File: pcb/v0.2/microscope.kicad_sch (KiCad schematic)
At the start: 26 parts, among them IC1 AL8860QMP-13, J1 Conn_01x02_Socket, J3 Conn_01x03_Socket, U1 OP07CDR, U2 NE555DR, U3 L78L05_SOT89, U4 Solder Pad, U5 Solder Pad

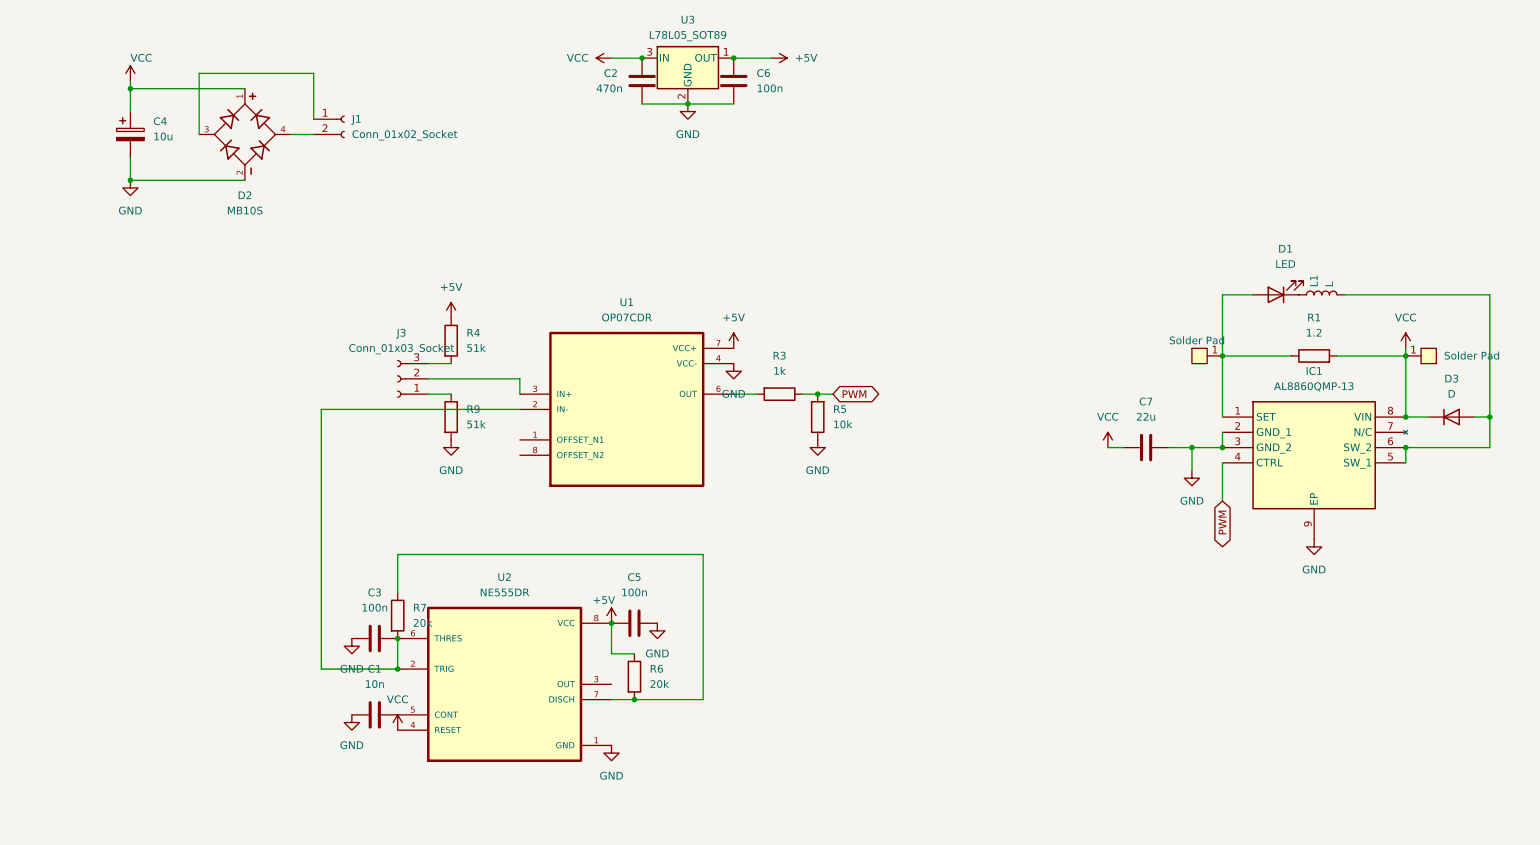
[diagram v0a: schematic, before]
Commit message: v0.2 pcb finished
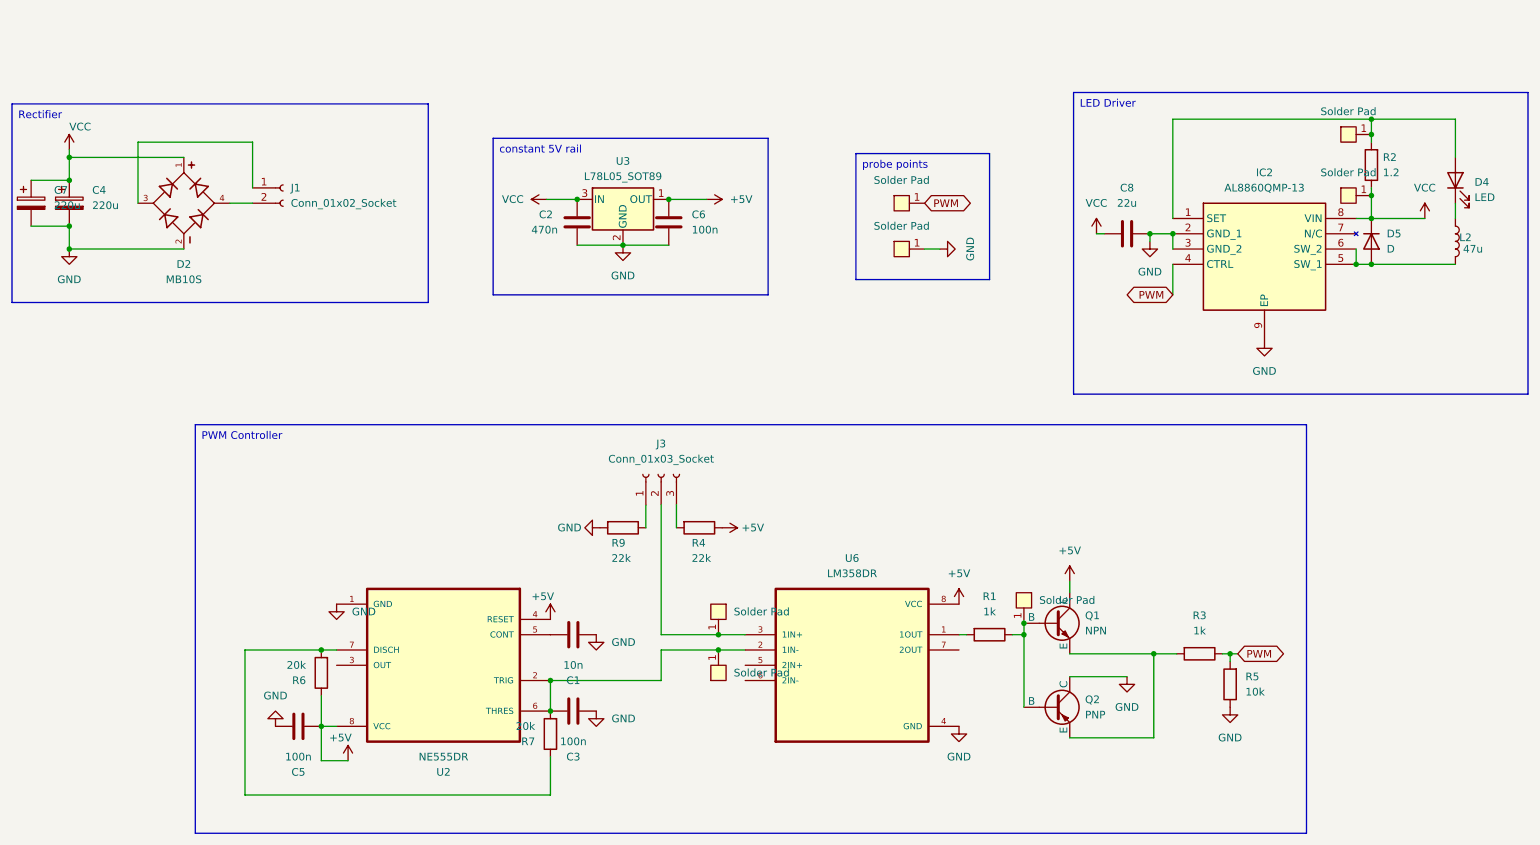
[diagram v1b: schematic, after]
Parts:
- removed C7: 22u, Capacitor_SMD:C_0805_2012Metric, symbol Device:C
- removed D1: LED, LED_SMD:LED_PLCC_2835, symbol Device:LED
- removed D3: D, Diode_SMD:D_SOD-323, symbol Device:D
- removed IC1: AL8860QMP-13, KiCad:SOP65P490X110-9N, symbol AL8860QMP-13:AL8860QMP-13
- removed L1: L, Inductor_SMD:L_1210_3225Metric, symbol Device:L
- removed U1: OP07CDR, OP07CDR:SOIC127P599X175-8N, symbol OP07CDR:OP07CDR
- added C7: 220u, Capacitor_THT:CP_Radial_D6.3mm_P2.50mm, symbol Device:C_Polarized
- added C8: 22u, Capacitor_SMD:C_0805_2012Metric, symbol Device:C
- added D4: LED, LED_SMD:LED_PLCC_2835, symbol Device:LED
- added D5: D, Diode_SMD:D_SOD-323, symbol Device:D
- added IC2: AL8860QMP-13, KiCad:SOP65P490X110-9N, symbol AL8860QMP-13:AL8860QMP-13
- added L2: 47u, Inductor_SMD:L_1210_3225Metric, symbol Device:L
- added Q1: NPN, custom_components:custom_SOT-23-3, symbol Simulation_SPICE:NPN
- added Q2: PNP, custom_components:custom_SOT-23-3, symbol Simulation_SPICE:PNP
- added R2: 1.2, Resistor_SMD:R_0603_1608Metric, symbol Device:R
- added U1, U10, U7, U8, U9: Solder Pad, custom_components:SolderPad_3x3mm, symbol custom_components:SolderPad
- added U6: LM358DR, LM358DR:SOIC127P599X175-8N, symbol LM358DR:LM358DR
- C1, C2, C3, C5, C6: footprint Capacitor_SMD:C_0805_2012Metric -> Capacitor_SMD:C_0603_1608Metric
- C4: value 10u -> 220u; footprint Capacitor_SMD:C_0805_2012Metric -> Capacitor_THT:CP_Radial_D6.3mm_P2.50mm; now left out of the parts list
- D2: Check_prices https://www.snapeda.com/parts/MB10S/MPD/view-part/?ref=eda -> https://www.snapeda.com/parts/MB10S/Onsemi/view-part/?ref=e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; LCSC (none) -> C2488; MF MDD -> ON Semiconductor; Package None -> SOIC-4 ON Semiconductor; SnapEDA_Link https://www.snapeda.com/parts/MB10S/MPD/view-part/?ref=snap -> https://www.snapeda.com/parts/MB10S/Onsemi/view-part/?ref=s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
- J1, J3, U4, U5: now left out of the parts list
- R1: value 1.2 -> 1k; footprint Resistor_SMD:R_0805_2012Metric -> Resistor_SMD:R_0603_1608Metric
- R3, R5, R6, R7: footprint Resistor_SMD:R_0805_2012Metric -> Resistor_SMD:R_0603_1608Metric
- R4, R9: value 51k -> 22k; footprint Resistor_SMD:R_0805_2012Metric -> Resistor_SMD:R_0603_1608Metric
- U2: LCSC (none) -> C7593
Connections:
- net +5V: now also U2.4 (RESET), Q1.1 (C), U6.8 (VCC)
- net GND: now also U4.1, C7.2, C8.2, IC2.2 (GND_1), IC2.3 (GND_2), IC2.9 (EP), Q2.1 (C), U6.4 (GND)
- net PWM: now also IC2.4 (CTRL), U1.1
- net VCC: now also C7.1, C8.1, D5.1 (K), IC2.8 (VIN), R2.1, U9.1; no longer R1.2, U2.4 (RESET), U5.1
- net at C3.1, R7.2, U2.2 (TRIG)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: now also U6.2 (1IN-), U8.1
- net at R1.1: now also Q1.2 (B), Q2.2 (B), U10.1; no longer U4.1
- net at J3.2 (Pin_2): now also U6.3 (1IN+), U7.1
- net at R3.2: now also Q1.3 (E), Q2.3 (E)
- new net: D4.2 (A), IC2.1 (SET), R2.2, U5.1
- new net: D5.2 (A), IC2.5 (SW_1), IC2.6 (SW_2), L2.2
- new net: D4.1 (K), L2.1
- new net: R1.2, U6.1 (1OUT)
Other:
- moved on the sheet: C1, C2, C3, C4, C5, C6, D2, J1, J3, R3, R4, R5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
